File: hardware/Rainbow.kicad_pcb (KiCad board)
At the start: 2 copper layers, 63.3 x 47.9 mm, 24 parts, among them J1 PICKit3, J2 UART, J3 BARREL_JACK, J4 HC-05, J5 RGB, Q1 Q_NMOS_GDS, Q2 Q_NMOS_GDS, Q3 Q_NMOS_GDS, SW1 SWITCH, U1 PIC16F15325, U2 MIC4574-5.0YN

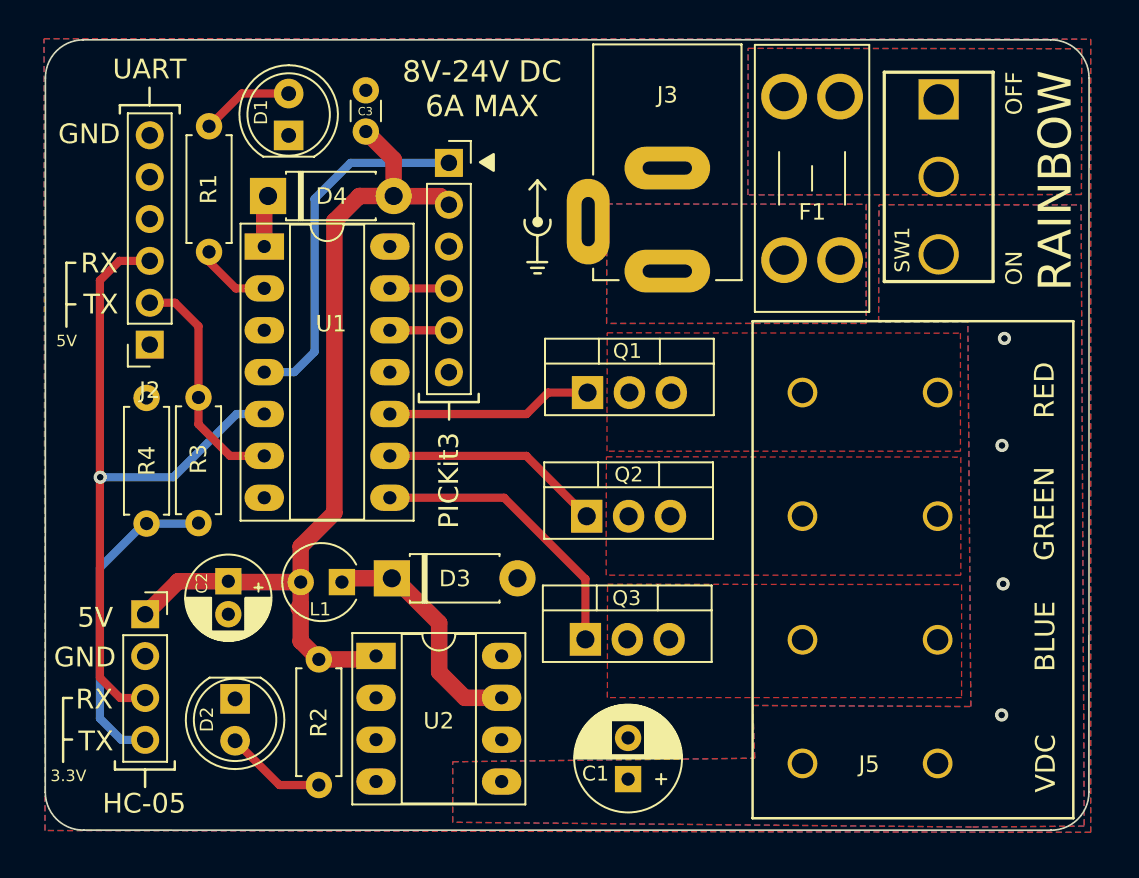
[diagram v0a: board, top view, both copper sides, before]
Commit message: Generate gerbers
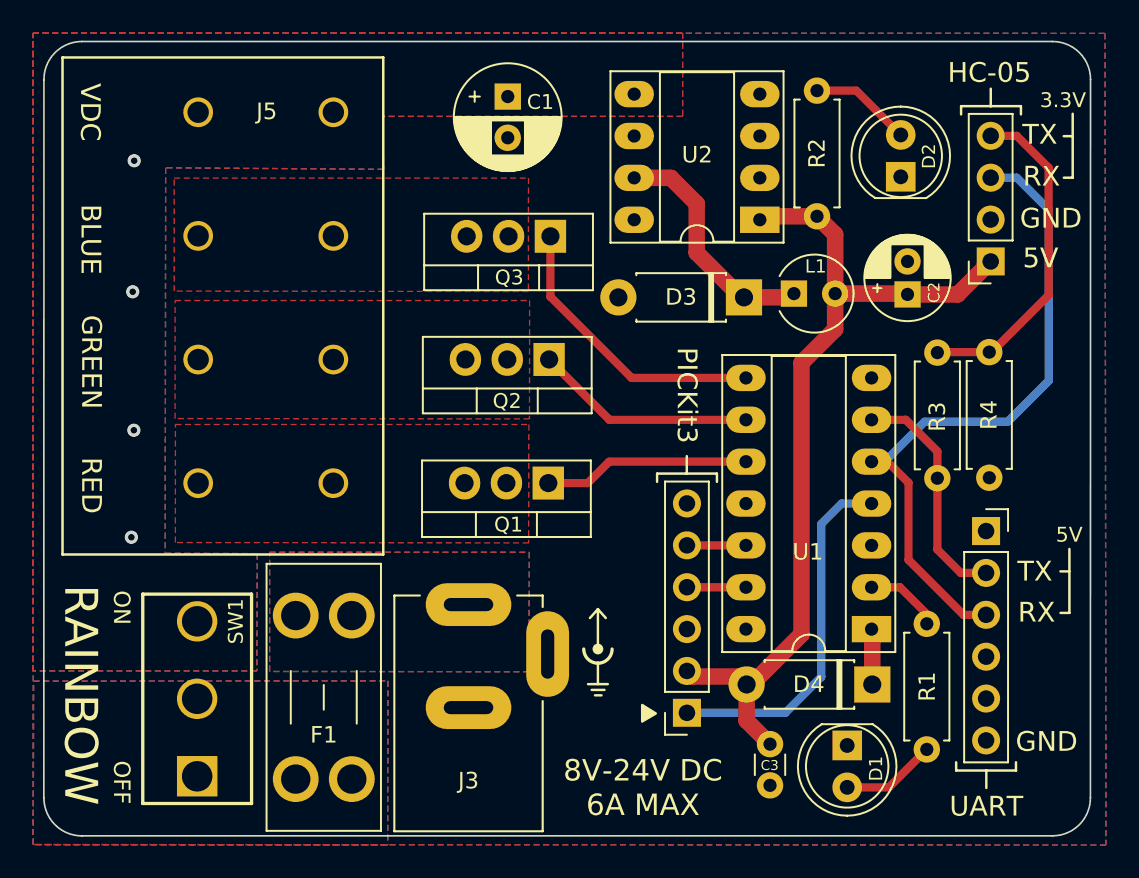
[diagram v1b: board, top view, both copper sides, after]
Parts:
- moved J4 55.6 mm to (169.3, 76.8), turned to 180 degrees
- moved SW1 55.0 mm to (121.1, 103.3), turned to 180 degrees
- moved R4 52.2 mm to (169.2, 82.3), turned to -90 degrees
- moved J2 52.0 mm to (169.0, 93.2), turned to 0 degrees
- moved D2 51.3 mm to (163.8, 71.7), turned to 90 degrees
- moved D1 50.2 mm to (160.6, 106.2), turned to -90 degrees
- moved J3 49.2 mm to (137.6, 111.4), turned to 90 degrees
- moved R1 49.0 mm to (165.4, 98.8), turned to -90 degrees
- moved J5 48.7 mm to (129.4, 67.8), turned to -90 degrees
- moved D4 47.1 mm to (162.1, 102.5), turned to 180 degrees
- moved R3 45.1 mm to (166.0, 90.0), turned to 90 degrees
- moved C2 44.7 mm to (164.2, 78.8), turned to 90 degrees
- moved C3 44.5 mm to (155.9, 106.1), turned to -90 degrees
- moved U1 43.5 mm to (162.1, 99.1), turned to 180 degrees
- moved C1 42.0 mm to (140.0, 66.8), turned to -90 degrees
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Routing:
- net RX: track 42.4 -> 41.0 mm, vias 1 -> 0
- net +5V: track 54.0 -> 53.0 mm
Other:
- board size 63.3 x 47.9 mm -> 63.5 x 48.2 mm
